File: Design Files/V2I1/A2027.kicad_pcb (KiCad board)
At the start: 2 copper layers, 78 parts, among them J1 Screw_Terminal_01x02, J3 Conn_02x03_Top_Bottom, J4 Conn_01x05_Pin, J6 Conn_01x02_Pin, J7 Conn_01x04_Pin, Q1 BSS138, Q2 BC857, Q3 BSS138, Q4 BC857, SW1 SW_SPDT, U1 TPS560200, U2 USBLC6-2SC6, U4 STM32F103C8T6, U5 LM1117MP-3.3, U6 DS3232M, U8 24LC256, Y1 16MHz

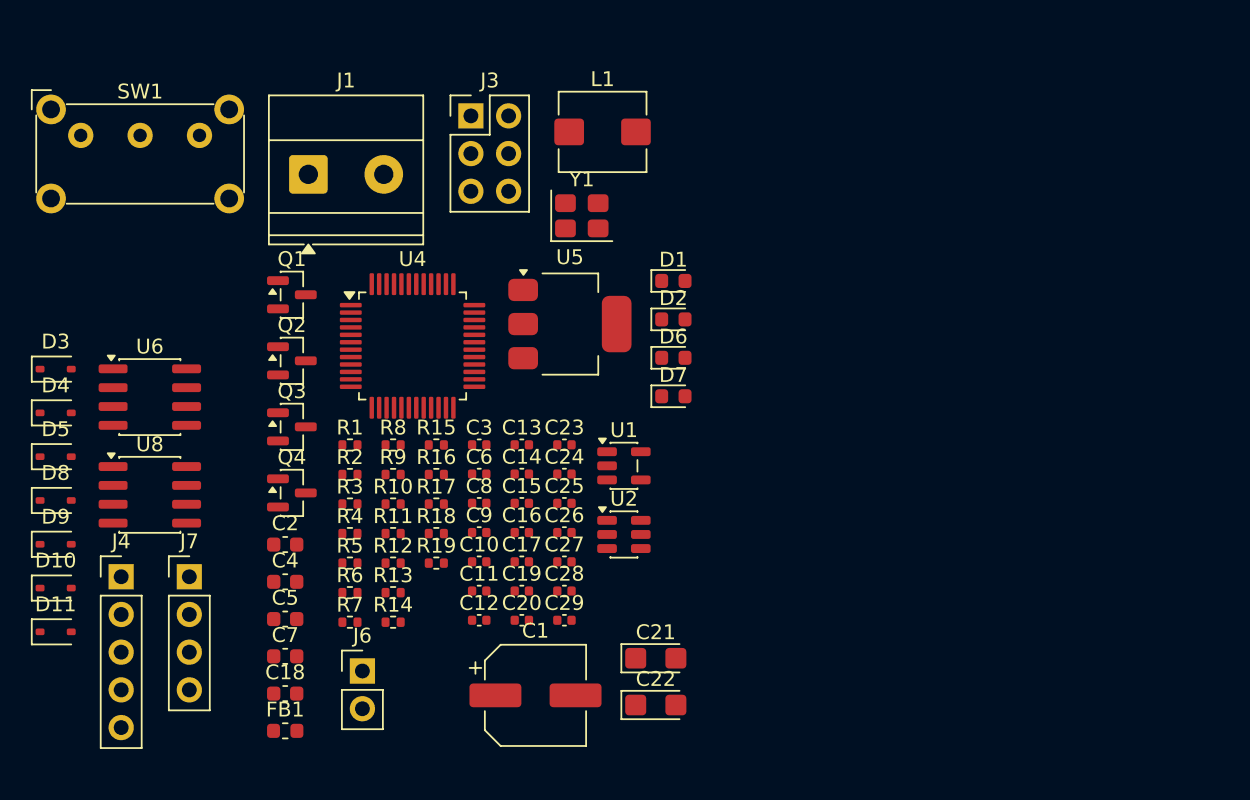
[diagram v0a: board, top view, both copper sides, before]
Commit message: master :: update schmea
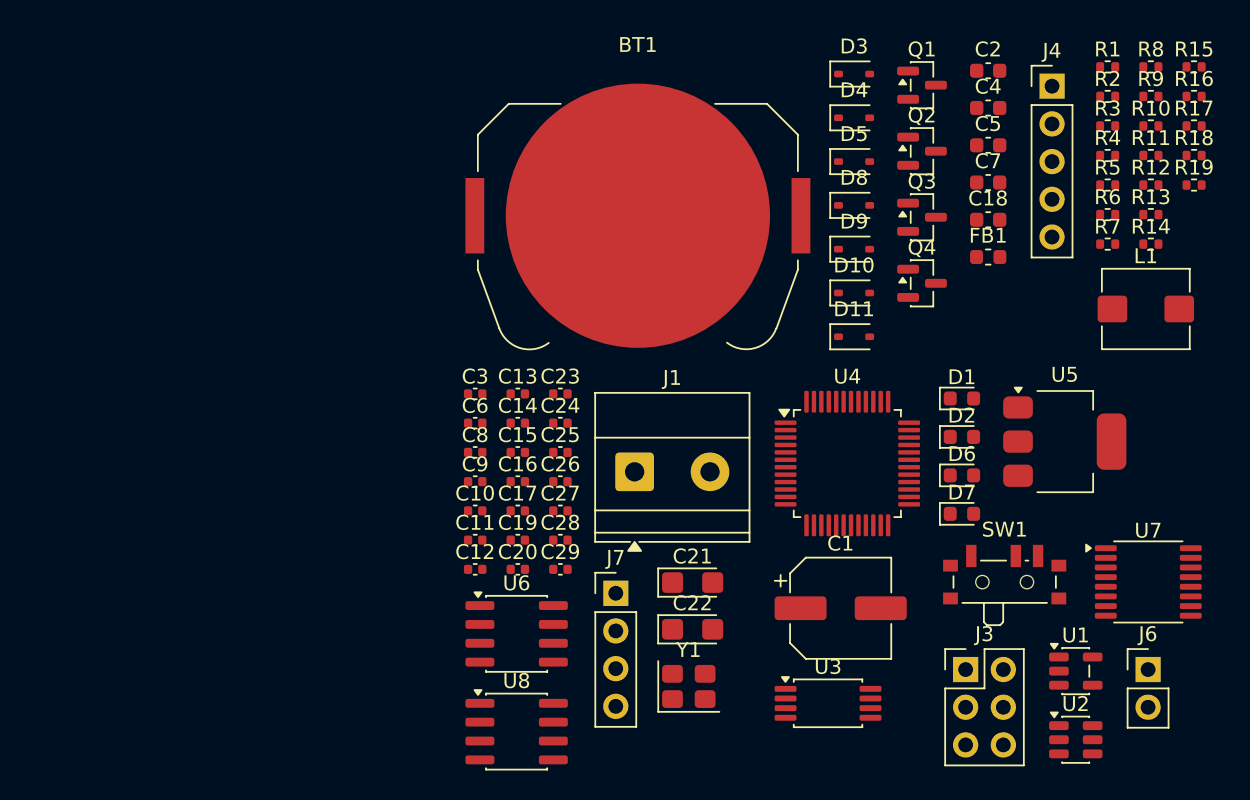
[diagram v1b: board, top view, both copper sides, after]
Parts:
- added BT1: 3.0V, Battery:BatteryHolder_Keystone_3034_1x20mm, F.Cu at (117.4, 89.0)
- added U3: TPS2113A, Package_SO:TSSOP-8_4.4x3mm_P0.65mm, F.Cu at (130.2, 121.9)
- added U7: MAX3232, Package_SO:TSSOP-16_4.4x5mm_P0.65mm, F.Cu at (151.8, 113.7)
- SW1: footprint Button_Switch_THT:SW_E-Switch_EG1224_SPDT_Angled -> Button_Switch_SMD:SW_SPDT_PCM12
- moved J4 70.9 mm to (145.3, 80.3)
- moved SW1 69.0 mm to (142.1, 113.4)
- moved D10 57.3 mm to (132.0, 94.2)
- moved D11 57.3 mm to (132.0, 97.2)
- moved D3 57.3 mm to (132.0, 79.5)
- moved D4 57.3 mm to (132.0, 82.4)
- moved D5 57.3 mm to (132.0, 85.4)
- moved D8 57.3 mm to (132.0, 88.3)
- moved D9 57.3 mm to (132.0, 91.3)
- moved C18 57.1 mm to (141.0, 89.3)
- moved C2 57.1 mm to (141.0, 79.3)
- moved C4 57.1 mm to (141.0, 81.8)
- moved C7 57.1 mm to (141.0, 86.8)
- moved C5 57.1 mm to (141.0, 84.3)
- moved FB1 57.1 mm to (141.0, 91.8)
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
